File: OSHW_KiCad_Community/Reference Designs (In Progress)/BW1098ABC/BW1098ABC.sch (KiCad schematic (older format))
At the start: 10 parts

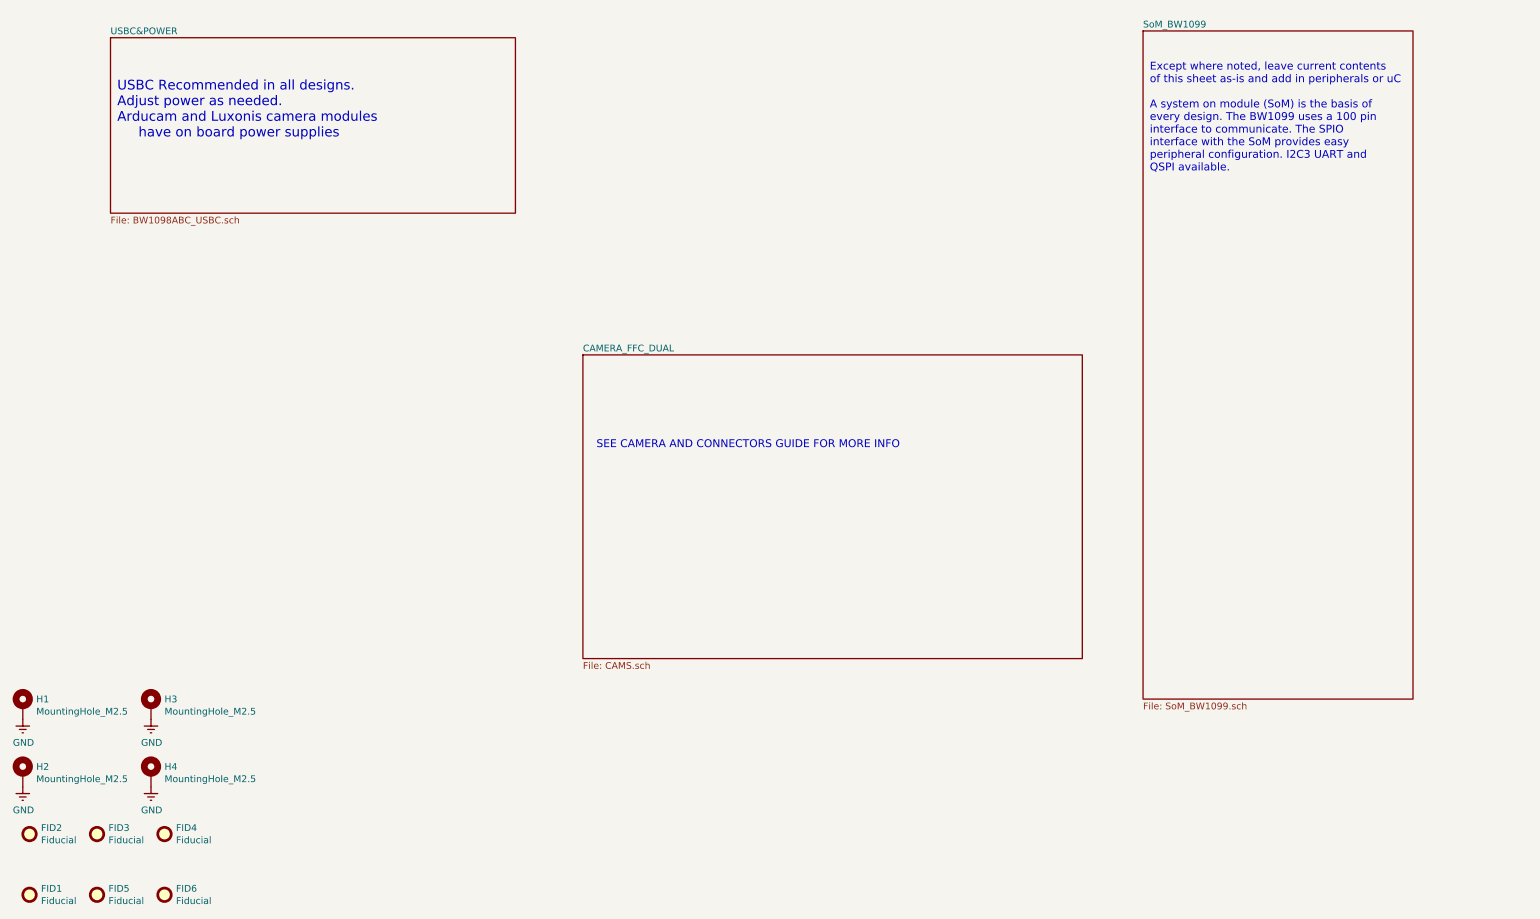
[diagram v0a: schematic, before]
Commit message: layout
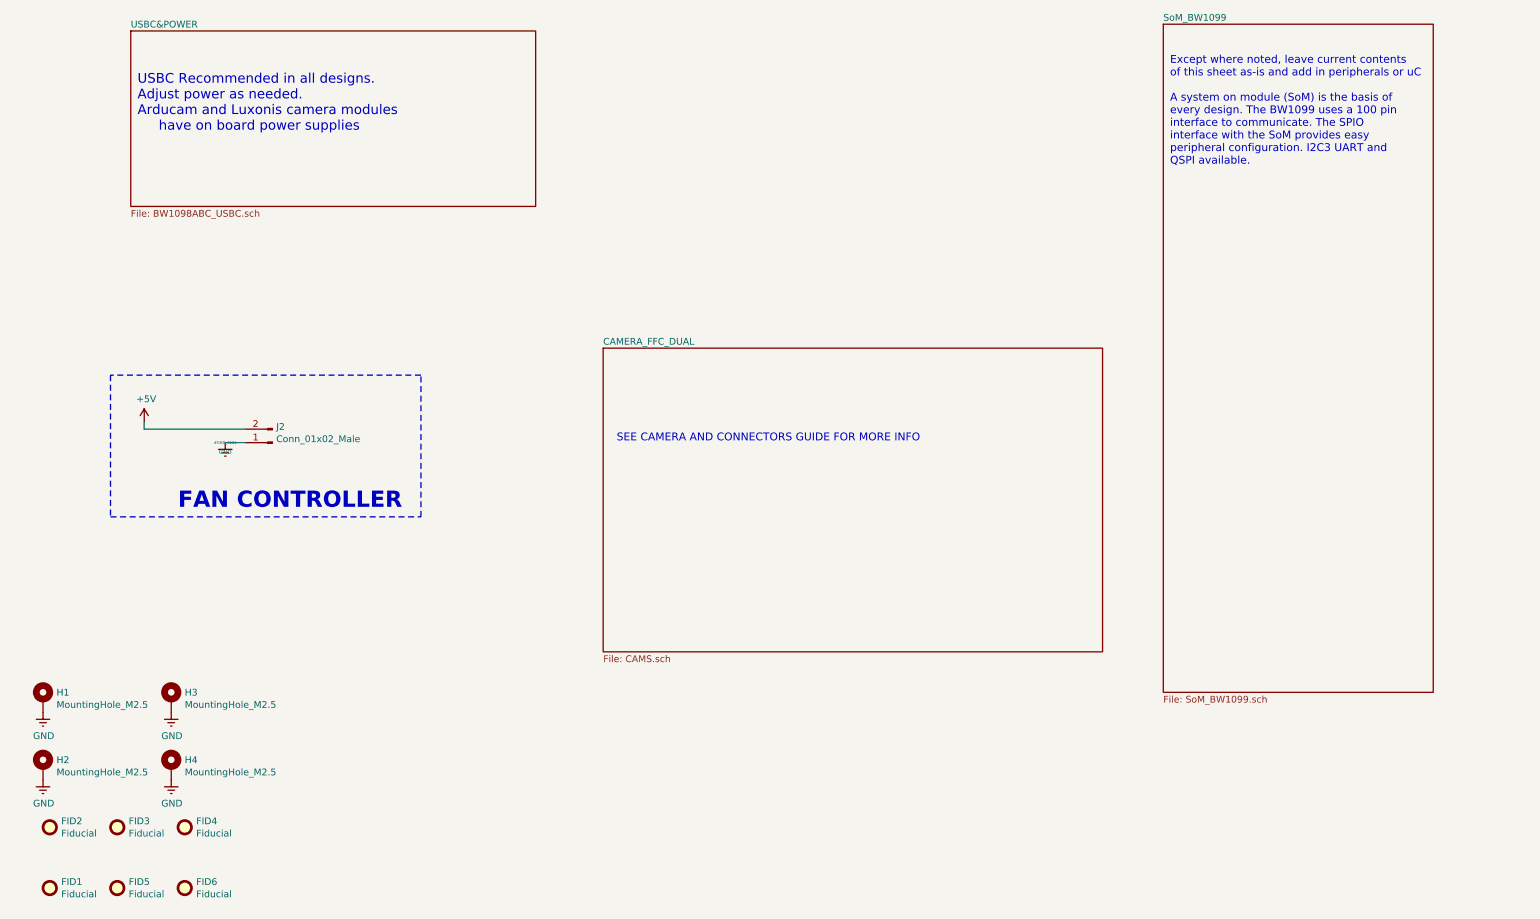
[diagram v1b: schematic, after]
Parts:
- added J2: Conn_01x02_Male, Connector_PinHeader_2.54mm:PinHeader_1x02_P2.54mm_Vertical, symbol Connector:Conn_01x02_Male
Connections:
- net Earth: now also J2.1 (Pin_1)
- new net +5V: J2.2 (Pin_2)
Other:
- note added: "FAN CONTROLLER"
- moved on the sheet: FID1, FID2, FID3, FID4, FID5, FID6, H1, H2, H3, H4
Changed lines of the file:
@@
 $EndDescr
 $Sheet
-S 8950 1000 2000 4950
+S 9100 950  2000 4950
 U 5FF8D9B2
 F0 "SoM_BW1099" 50
@@
 L Mechanical:Fiducial FID1
 U 1 1 6049A903
-P 700 7400
-F 0 "FID1" H 785 7446 50  0000 L CNN
-F 1 "Fiducial" H 785 7355 50  0000 L CNN
-F 2 "Fiducial:Fiducial_1mm_Mask2mm" H 700 7400 50  0001 C CNN
-F 3 "~" H 700 7400 50  0001 C CNN
-	1    700  7400
+P 850 7350
+F 0 "FID1" H 935 7396 50  0000 L CNN
+F 1 "Fiducial" H 935 7305 50  0000 L CNN
+F 2 "Fiducial:Fiducial_1mm_Mask2mm" H 850 7350 50  0001 C CNN
+F 3 "~" H 850 7350 50  0001 C CNN
+	1    850  7350
 	1    0    0    -1
 $EndComp
@@
 L Mechanical:Fiducial FID2
 U 1 1 5FF51DEB
-P 700 6950
-F 0 "FID2" H 785 6996 50  0000 L CNN
-F 1 "Fiducial" H 785 6905 50  0000 L CNN
-F 2 "Fiducial:Fiducial_1mm_Mask2mm" H 700 6950 50  0001 C CNN
-F 3 "~" H 700 6950 50  0001 C CNN
-	1    700  6950
+P 850 6900
+F 0 "FID2" H 935 6946 50  0000 L CNN
+F 1 "Fiducial" H 935 6855 50  0000 L CNN
+F 2 "Fiducial:Fiducial_1mm_Mask2mm" H 850 6900 50  0001 C CNN
+F 3 "~" H 850 6900 50  0001 C CNN
+	1    850  6900
 	1    0    0    -1
 $EndComp
@@
 L Mechanical:Fiducial FID3
 U 1 1 6049A905
-P 1200 6950
-F 0 "FID3" H 1285 6996 50  0000 L CNN
-F 1 "Fiducial" H 1285 6905 50  0000 L CNN
-F 2 "Fiducial:Fiducial_1mm_Mask2mm" H 1200 6950 50  0001 C CNN
-F 3 "~" H 1200 6950 50  0001 C CNN
-	1    1200 6950
+P 1350 6900
+F 0 "FID3" H 1435 6946 50  0000 L CNN
+F 1 "Fiducial" H 1435 6855 50  0000 L CNN
+F 2 "Fiducial:Fiducial_1mm_Mask2mm" H 1350 6900 50  0001 C CNN
+F 3 "~" H 1350 6900 50  0001 C CNN
+	1    1350 6900
 	1    0    0    -1
 $EndComp
@@
 L Mechanical:Fiducial FID4
 U 1 1 6049A906
-P 1700 6950
-F 0 "FID4" H 1785 6996 50  0000 L CNN
-F 1 "Fiducial" H 1785 6905 50  0000 L CNN
-F 2 "Fiducial:Fiducial_1mm_Mask2mm" H 1700 6950 50  0001 C CNN
-F 3 "~" H 1700 6950 50  0001 C CNN
-	1    1700 6950
+P 1850 6900
+F 0 "FID4" H 1935 6946 50  0000 L CNN
+F 1 "Fiducial" H 1935 6855 50  0000 L CNN
+F 2 "Fiducial:Fiducial_1mm_Mask2mm" H 1850 6900 50  0001 C CNN
+F 3 "~" H 1850 6900 50  0001 C CNN
+	1    1850 6900
 	1    0    0    -1
 $EndComp
@@
 L Mechanical:Fiducial FID5
 U 1 1 6049A907
-P 1200 7400
-F 0 "FID5" H 1285 7446 50  0000 L CNN
-F 1 "Fiducial" H 1285 7355 50  0000 L CNN
-F 2 "Fiducial:Fiducial_1mm_Mask2mm" H 1200 7400 50  0001 C CNN
-F 3 "~" H 1200 7400 50  0001 C CNN
-	1    1200 7400
+P 1350 7350
+F 0 "FID5" H 1435 7396 50  0000 L CNN
+F 1 "Fiducial" H 1435 7305 50  0000 L CNN
+F 2 "Fiducial:Fiducial_1mm_Mask2mm" H 1350 7350 50  0001 C CNN
+F 3 "~" H 1350 7350 50  0001 C CNN
+	1    1350 7350
 	1    0    0    -1
 $EndComp
@@
 L Mechanical:Fiducial FID6
 U 1 1 600C0C22
-P 1700 7400
-F 0 "FID6" H 1785 7446 50  0000 L CNN
-F 1 "Fiducial" H 1785 7355 50  0000 L CNN
-F 2 "Fiducial:Fiducial_1mm_Mask2mm" H 1700 7400 50  0001 C CNN
-F 3 "~" H 1700 7400 50  0001 C CNN
-	1    1700 7400
+P 1850 7350
+F 0 "FID6" H 1935 7396 50  0000 L CNN
+F 1 "Fiducial" H 1935 7305 50  0000 L CNN
+F 2 "Fiducial:Fiducial_1mm_Mask2mm" H 1850 7350 50  0001 C CNN
+F 3 "~" H 1850 7350 50  0001 C CNN
+	1    1850 7350
 	1    0    0    -1
 $EndComp
@@
 L BW1098ABC-rescue:Mechanical_MountingHole_Pad-depthAI_sch H1
 U 1 1 600C0C23
-P 650 6000
-F 0 "H1" H 750 6049 50  0000 L CNN
-F 1 "MountingHole_M2.5" H 750 5958 50  0000 L CNN
-F 2 "Mounting_Wuerth:Mounting_Wuerth_WA-SMSI-M2_H3mm_9774030243" H 650 6000 50  0001 C CNN
-F 3 "" H 650 6000 50  0001 C CNN
-	1    650  6000
+P 800 5950
+F 0 "H1" H 900 5999 50  0000 L CNN
+F 1 "MountingHole_M2.5" H 900 5908 50  0000 L CNN
+F 2 "Mounting_Wuerth:Mounting_Wuerth_WA-SMSI-M2_H3mm_9774030243" H 800 5950 50  0001 C CNN
+F 3 "" H 800 5950 50  0001 C CNN
+	1    800  5950
 	1    0    0    -1
 $EndComp
@@
 L BW1098ABC-rescue:Mechanical_MountingHole_Pad-depthAI_sch H2
 U 1 1 600C0C24
-P 650 6500
-F 0 "H2" H 750 6549 50  0000 L CNN
-F 1 "MountingHole_M2.5" H 750 6458 50  0000 L CNN
-F 2 "Mounting_Wuerth:Mounting_Wuerth_WA-SMSI-M2_H3mm_9774030243" H 650 6500 50  0001 C CNN
-F 3 "" H 650 6500 50  0001 C CNN
-	1    650  6500
+P 800 6450
+F 0 "H2" H 900 6499 50  0000 L CNN
+F 1 "MountingHole_M2.5" H 900 6408 50  0000 L CNN
+F 2 "Mounting_Wuerth:Mounting_Wuerth_WA-SMSI-M2_H3mm_9774030243" H 800 6450 50  0001 C CNN
+F 3 "" H 800 6450 50  0001 C CNN
+	1    800  6450
 	1    0    0    -1
 $EndComp
@@
 L BW1098ABC-rescue:Mechanical_MountingHole_Pad-depthAI_sch H4
 U 1 1 600C0C25
-P 1600 6500
-F 0 "H4" H 1700 6549 50  0000 L CNN
-F 1 "MountingHole_M2.5" H 1700 6458 50  0000 L CNN
-F 2 "Mounting_Wuerth:Mounting_Wuerth_WA-SMSI-M2_H3mm_9774030243" H 1600 6500 50  0001 C CNN
-F 3 "" H 1600 6500 50  0001 C CNN
-	1    1600 6500
+P 1750 6450
+F 0 "H4" H 1850 6499 50  0000 L CNN
+F 1 "MountingHole_M2.5" H 1850 6408 50  0000 L CNN
+F 2 "Mounting_Wuerth:Mounting_Wuerth_WA-SMSI-M2_H3mm_9774030243" H 1750 6450 50  0001 C CNN
+F 3 "" H 1750 6450 50  0001 C CNN
+	1    1750 6450
 	1    0    0    -1
 $EndComp
@@
 L BW1098ABC-rescue:Mechanical_MountingHole_Pad-depthAI_sch H3
 U 1 1 600C0C26
-P 1600 6000
-F 0 "H3" H 1700 6049 50  0000 L CNN
-F 1 "MountingHole_M2.5" H 1700 5958 50  0000 L CNN
-F 2 "Mounting_Wuerth:Mounting_Wuerth_WA-SMSI-M2_H3mm_9774030243" H 1600 6000 50  0001 C CNN
-F 3 "" H 1600 6000 50  0001 C CNN
-	1    1600 6000
+P 1750 5950
+F 0 "H3" H 1850 5999 50  0000 L CNN
+F 1 "MountingHole_M2.5" H 1850 5908 50  0000 L CNN
+F 2 "Mounting_Wuerth:Mounting_Wuerth_WA-SMSI-M2_H3mm_9774030243" H 1750 5950 50  0001 C CNN
+F 3 "" H 1750 5950 50  0001 C CNN
+	1    1750 5950
 	1    0    0    -1
 $EndComp
 $Sheet
-S 4800 3400 3700 2250
+S 4950 3350 3700 2250
 U 5FF8D2B3
 F0 "CAMERA_FFC_DUAL" 50
@@
 L power:Earth #PWR0107
 U 1 1 6106C817
-P 650 6100
-F 0 "#PWR0107" H 650 5850 50  0001 C CNN
-F 1 "GND" H 655 5927 50  0000 C CNN
-F 2 "" H 650 6100 50  0001 C CNN
-F 3 "" H 650 6100 50  0001 C CNN
-	1    650  6100
+P 800 6050
+F 0 "#PWR0107" H 800 5800 50  0001 C CNN
+F 1 "GND" H 805 5877 50  0000 C CNN
+F 2 "" H 800 6050 50  0001 C CNN
+F 3 "" H 800 6050 50  0001 C CNN
+	1    800  6050
 	1    0    0    -1
 $EndComp
@@
 L power:Earth #PWR0108
 U 1 1 6106D903
-P 1600 6100
-F 0 "#PWR0108" H 1600 5850 50  0001 C CNN
-F 1 "GND" H 1605 5927 50  0000 C CNN
-F 2 "" H 1600 6100 50  0001 C CNN
-F 3 "" H 1600 6100 50  0001 C CNN
-	1    1600 6100
+P 1750 6050
+F 0 "#PWR0108" H 1750 5800 50  0001 C CNN
+F 1 "GND" H 1755 5877 50  0000 C CNN
+F 2 "" H 1750 6050 50  0001 C CNN
+F 3 "" H 1750 6050 50  0001 C CNN
+	1    1750 6050
 	1    0    0    -1
 $EndComp
@@
 L power:Earth #PWR0109
 U 1 1 6106E6FC
-P 1600 6600
-F 0 "#PWR0109" H 1600 6350 50  0001 C CNN
-F 1 "GND" H 1605 6427 50  0000 C CNN
-F 2 "" H 1600 6600 50  0001 C CNN
-F 3 "" H 1600 6600 50  0001 C CNN
-	1    1600 6600
+P 1750 6550
+F 0 "#PWR0109" H 1750 6300 50  0001 C CNN
+F 1 "GND" H 1755 6377 50  0000 C CNN
+F 2 "" H 1750 6550 50  0001 C CNN
+F 3 "" H 1750 6550 50  0001 C CNN
+	1    1750 6550
 	1    0    0    -1
 $EndComp
@@
 L power:Earth #PWR0110
 U 1 1 6106EA7D
-P 650 6600
-F 0 "#PWR0110" H 650 6350 50  0001 C CNN
-F 1 "GND" H 655 6427 50  0000 C CNN
-F 2 "" H 650 6600 50  0001 C CNN
-F 3 "" H 650 6600 50  0001 C CNN
-	1    650  6600
+P 800 6550
+F 0 "#PWR0110" H 800 6300 50  0001 C CNN
+F 1 "GND" H 805 6377 50  0000 C CNN
+F 2 "" H 800 6550 50  0001 C CNN
+F 3 "" H 800 6550 50  0001 C CNN
+	1    800  6550
 	1    0    0    -1
 $EndComp
 $Sheet
-S 1300 1050 3000 1300
+S 1450 1000 3000 1300
 U 60483E6B
 F0 "USBC&POWER" 50
 F1 "BW1098ABC_USBC.sch" 50
 $EndSheet
-Text Notes 4900 4100 0    58   ~ 0
+Text Notes 5050 4050 0    58   ~ 0
 SEE CAMERA AND CONNECTORS GUIDE FOR MORE INFO\n
-Text Notes 9000 2050 0    58   ~ 0
+Text Notes 9150 2000 0    58   ~ 0
 Except where noted, leave current contents\nof this sheet as-is and add in peripherals or uC\n\nA system on module (SoM) is the basis of \nevery design. The BW1099 uses a 100 pin\ninterface to communicate. The SPIO \ninterface with the SoM provides easy \nperipheral configuration. I2C3 UART and \nQSPI available.
-Text Notes 1350 1800 0    72   ~ 0
+Text Notes 1500 1750 0    72   ~ 0
 USBC Recommended in all designs. \nAdjust power as needed. \nArducam and Luxonis camera modules \n     have on board power supplies
+$Comp
+L power:Earth #GND_?
+U 1 1 60A13627
+P 2150 4050
+AR Path="/5FD7EFCB/60A13627" Ref="#GND_?"  Part="1"
+AR Path="/604AEAFA/60A13627" Ref="#GND_?"  Part="1"
+AR Path="/60483E6B/60A13627" Ref="#GND_?"  Part="1"
+AR Path="/60A13627" Ref="#GND_0101"  Part="1"
+F 0 "#GND_0101" H 2150 4050 20  0000 C CNN
+F 1 "GND" H 2150 3980 30  0000 C CNN
+F 2 "" H 2150 4050 70  0000 C CNN
+F 3 "" H 2150 4050 70  0000 C CNN
+	1    2150 4050
+	1    0    0    -1
+$EndComp
+Text Notes 1800 4550 0    120  ~ 24
+FAN CONTROLLER
+Wire Wire Line
+	2300 4050 2150 4050
+$Comp
+L power:+5V #PWR?
+U 1 1 60A1362F
+P 1550 3900
+AR Path="/60483E6B/60A1362F" Ref="#PWR?"  Part="1"
+AR Path="/60A1362F" Ref="#PWR0111"  Part="1"
+F 0 "#PWR0111" H 1550 3750 50  0001 C CNN
+F 1 "+5V" H 1565 4073 50  0000 C CNN
+F 2 "" H 1550 3900 50  0001 C CNN
+F 3 "" H 1550 3900 50  0001 C CNN
+	1    1550 3900
+	1    0    0    -1
+$EndComp
+Wire Wire Line
+	1550 3950 1550 3900
+Wire Wire Line
+	1550 3950 2300 3950
+Wire Notes Line
+	3600 3550 1300 3550
+Wire Notes Line
+	1300 3550 1300 4600
+Wire Notes Line
+	1300 4600 3600 4600
+Wire Notes Line
+	3600 4600 3600 3550
+$Comp
+L Connector:Conn_01x02_Male J?
+U 1 1 60A1363B
+P 2500 4050
+AR Path="/60483E6B/60A1363B" Ref="J?"  Part="1"
+AR Path="/60A1363B" Ref="J2"  Part="1"
+F 0 "J2" H 2472 3932 50  0000 R CNN
+F 1 "Conn_01x02_Male" H 2472 4023 50  0000 R CNN
+F 2 "Connector_PinHeader_2.54mm:PinHeader_1x02_P2.54mm_Vertical" H 2500 4050 50  0001 C CNN
+F 3 "~" H 2500 4050 50  0001 C CNN
+	1    2500 4050
+	-1   0    0    1
+$EndComp
 $EndSCHEMATC
